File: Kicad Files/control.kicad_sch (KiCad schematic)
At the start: 61 parts, among them U46 74LS02, U47 74LS161, U48 SST39SF020, U49 SST39SF020, U50 SST39SF020

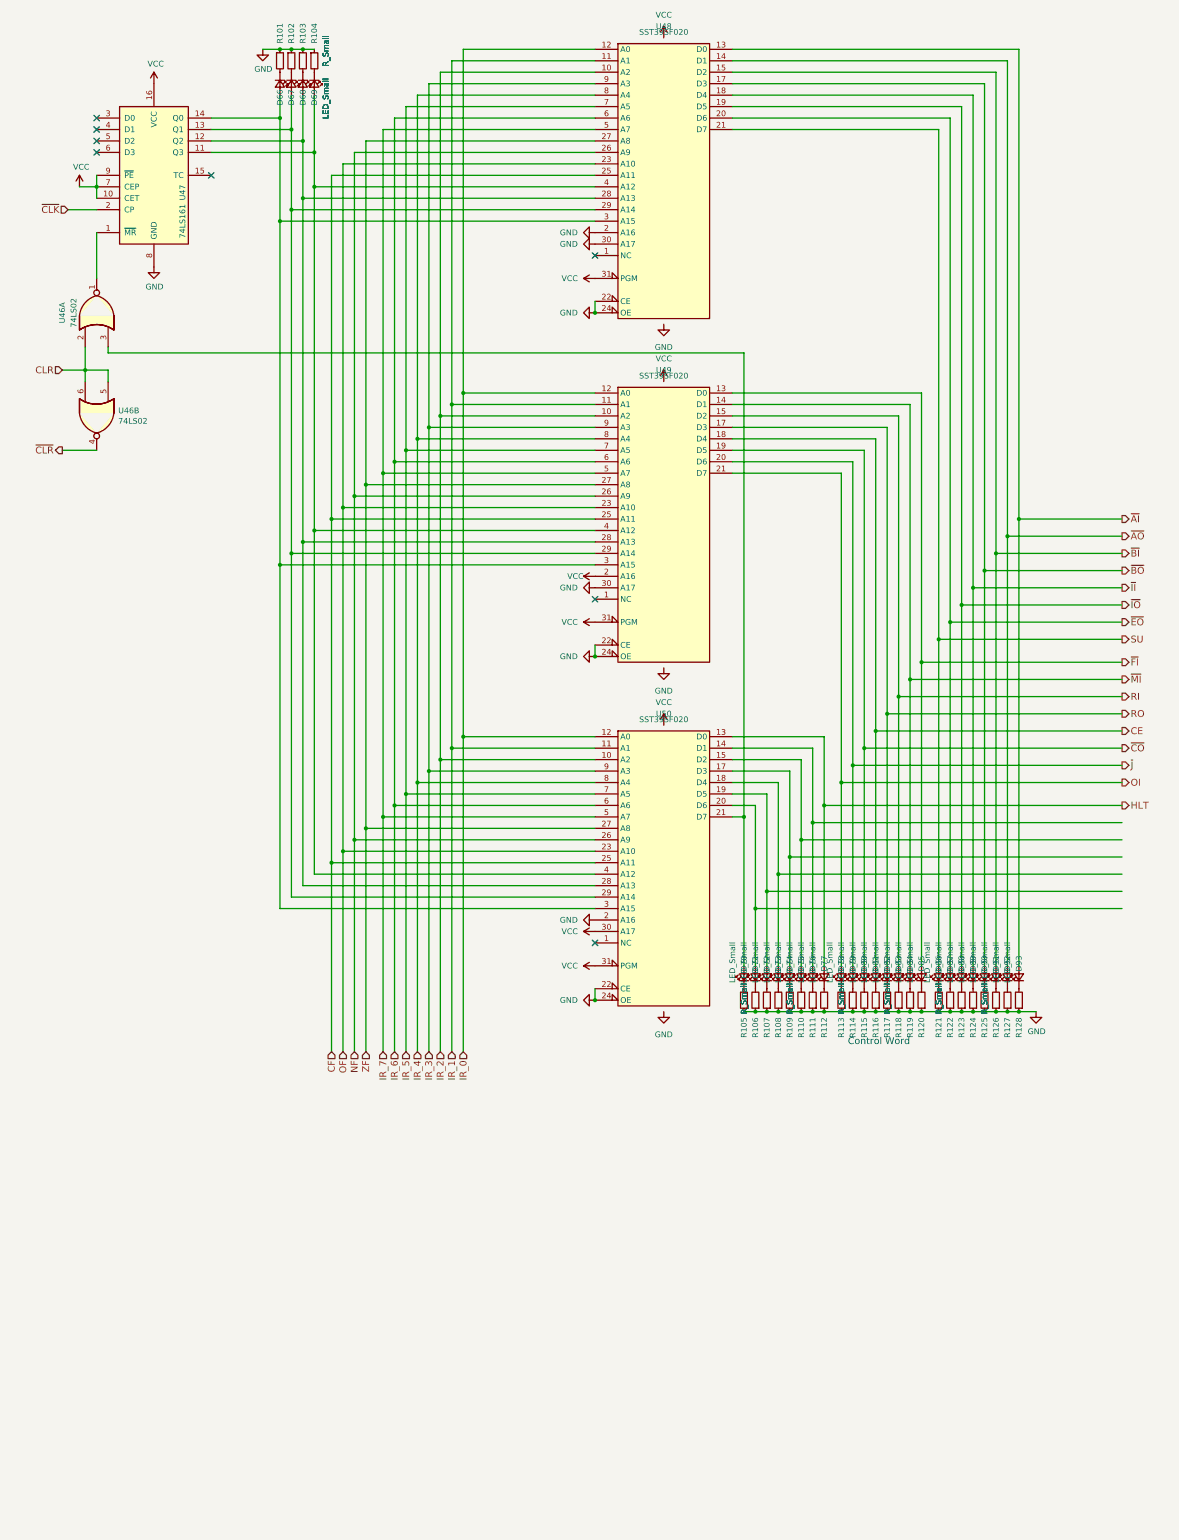
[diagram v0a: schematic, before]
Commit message: put it allll together
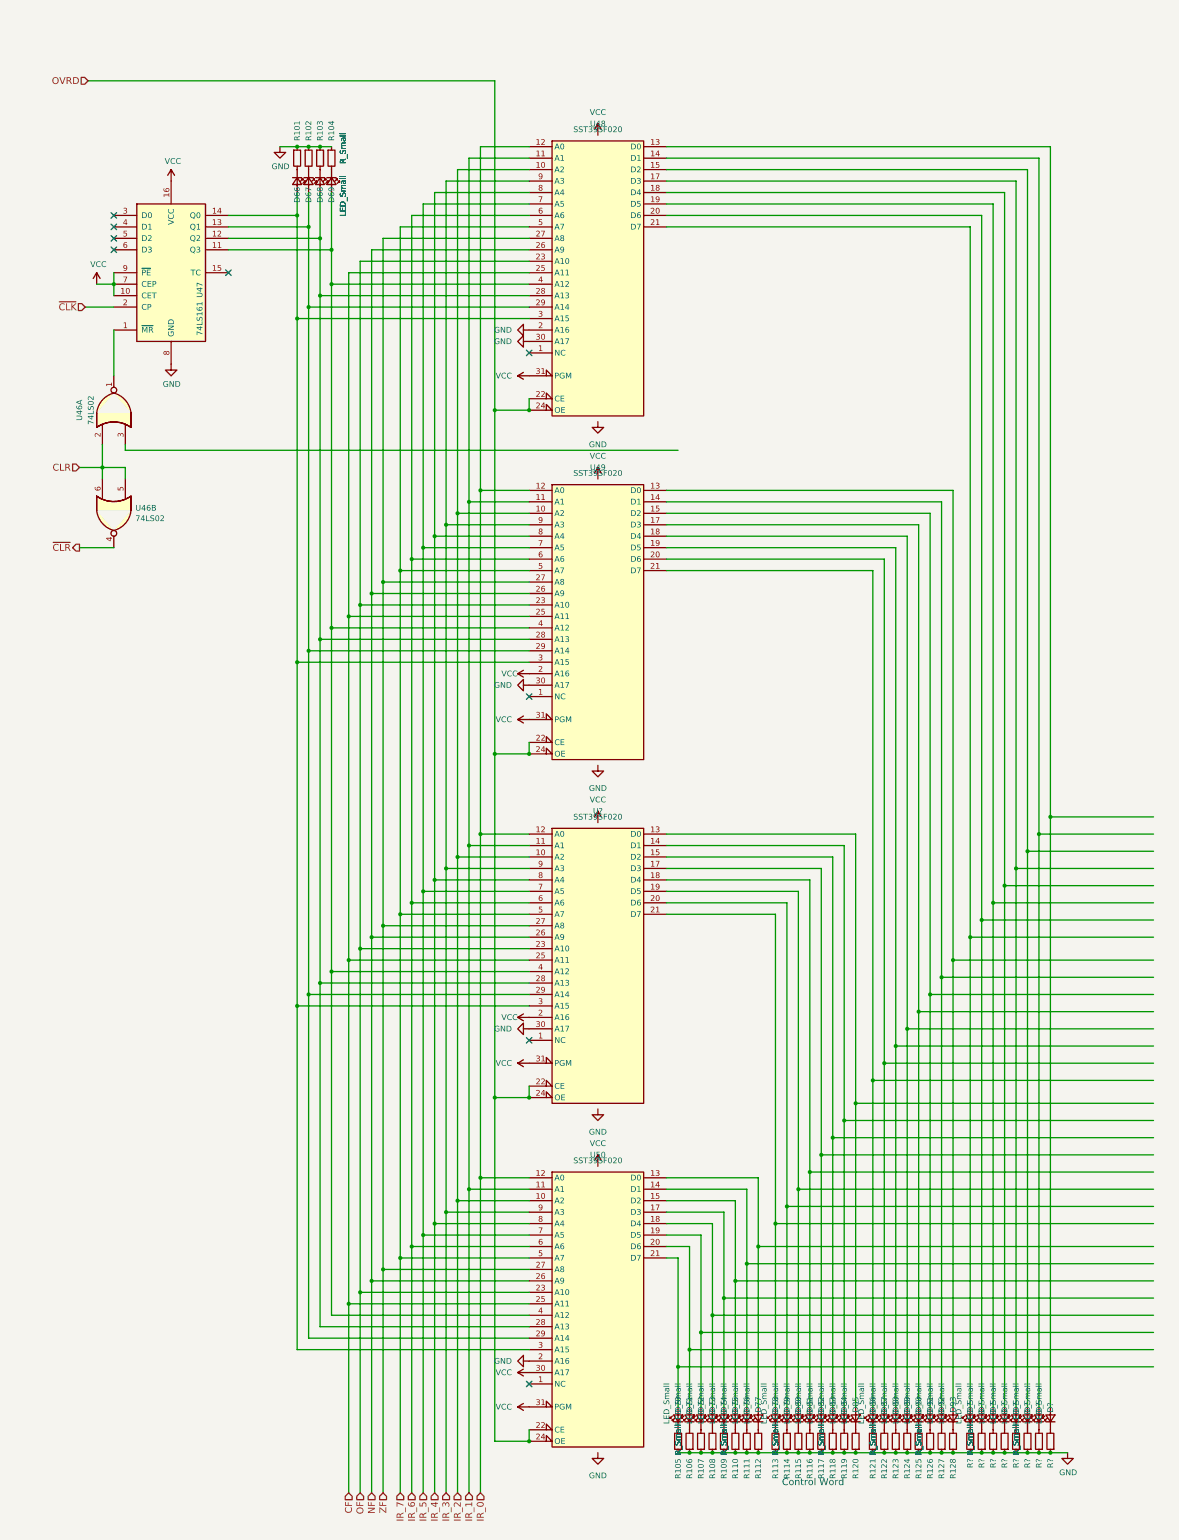
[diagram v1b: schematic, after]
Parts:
- added D? (x8): LED_Small, symbol Device:LED_Small
- added R? (x8): R_Small, symbol Device:R_Small
- added U?: SST39SF020, symbol Memory_Flash:SST39SF020
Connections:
- net CF: now also U?.25 (A11)
- net GND: now also R?.1, R?.1, R?.1, R?.1, R?.1, R?.1, R?.1, R?.1, U?.16 (GND), U?.30 (A17); no longer U48.22 (CE), U48.24 (OE), U49.22 (CE), U49.24 (OE), U50.22 (CE), U50.24 (OE)
- net IR_0: now also U?.12 (A0)
- net IR_1: now also U?.11 (A1)
- net IR_2: now also U?.10 (A2)
- net IR_3: now also U?.9 (A3)
- net IR_4: now also U?.8 (A4)
- net IR_5: now also U?.7 (A5)
- net IR_6: now also U?.6 (A6)
- net IR_7: now also U?.5 (A7)
- net NF: now also U?.26 (A9)
- net OF: now also U?.23 (A10)
- net VCC: now also U?.2 (A16), U?.31 (PGM), U?.32 (VCC)
- net ZF: now also U?.27 (A8)
- net at D69.2 (A), U47.11 (Q3), U48.4 (A12)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: now also U?.4 (A12)
- net at D68.2 (A), U47.12 (Q2), U48.28 (A13)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: now also U?.28 (A13)
- net at D67.2 (A), U47.13 (Q1), U48.29 (A14)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: now also U?.29 (A14)
- net at D66.2 (A), U47.14 (Q0), U48.3 (A15)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: now also U?.3 (A15)
- net at D70.2 (A), U50.21 (D7): no longer U46.3
- net CE: no longer names the net of D81.2 (A)
- net CE: now also U?.18 (D4); no longer U49.18 (D4)
- net HLT: no longer names the net of D77.2 (A), U50.13 (D0)
- net OI: no longer names the net of D78.2 (A)
- net OI: now also U?.21 (D7); no longer U49.21 (D7)
- net RI: no longer names the net of D83.2 (A)
- net RI: now also U?.15 (D2); no longer U49.15 (D2)
- net RO: no longer names the net of D82.2 (A)
- net RO: now also U?.17 (D3); no longer U49.17 (D3)
- net SU: no longer names the net of D86.2 (A)
- net SU: now also U49.21 (D7); no longer U48.21 (D7)
- net ~{AI}: no longer names the net of D93.2 (A)
- net ~{AI}: now also U49.13 (D0); no longer U48.13 (D0)
- net ~{AO}: no longer names the net of D92.2 (A)
- net ~{AO}: now also U49.14 (D1); no longer U48.14 (D1)
- net ~{BI}: no longer names the net of D91.2 (A)
- net ~{BI}: now also U49.15 (D2); no longer U48.15 (D2)
- net ~{BO}: no longer names the net of D90.2 (A)
- net ~{BO}: now also U49.17 (D3); no longer U48.17 (D3)
- net ~{CO}: no longer names the net of D80.2 (A)
- net ~{CO}: now also U?.19 (D5); no longer U49.19 (D5)
- net ~{EO}: no longer names the net of D87.2 (A)
- net ~{EO}: now also U49.20 (D6); no longer U48.20 (D6)
- net ~{FI}: no longer names the net of D85.2 (A)
- net ~{FI}: now also U?.13 (D0); no longer U49.13 (D0)
- net ~{II}: no longer names the net of D89.2 (A)
- net ~{II}: now also U49.18 (D4); no longer U48.18 (D4)
- net ~{IO}: no longer names the net of D88.2 (A)
- net ~{IO}: now also U49.19 (D5); no longer U48.19 (D5)
- net ~{J}: no longer names the net of D79.2 (A)
- net ~{J}: now also U?.20 (D6); no longer U49.20 (D6)
- net ~{MI}: no longer names the net of D84.2 (A)
- net ~{MI}: now also U?.14 (D1); no longer U49.14 (D1)
- new net: D?.1 (K), R?.2 (x8)
- new net: D?.2 (A), U48.13 (D0)
- new net: D?.2 (A), U48.21 (D7)
- new net: D?.2 (A), U48.19 (D5)
- new net: D?.2 (A), U48.15 (D2)
- new net: D?.2 (A), U48.14 (D1)
- new net: D?.2 (A), U48.20 (D6)
- new net: D?.2 (A), U48.17 (D3)
- new net: D?.2 (A), U48.18 (D4)
- new net OVRD: U48.22 (CE), U48.24 (OE), U49.22 (CE), U49.24 (OE), U50.22 (CE), U50.24 (OE), U?.22 (CE), U?.24 (OE)
- no-connect marks 8 -> 9
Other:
- moved on the sheet: D66, D67, D68, D69, D70, D71, D72, D73, D74, D75, D76, D77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
